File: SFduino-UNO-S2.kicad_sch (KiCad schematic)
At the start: 27 parts, among them J5 FPC 16p 0.5mm, SW1 SKHMQLE010, U1 SF32LB527UD6, U2 PY25Q128HA-WXH-IR, U8 CH334P, U9 CH343P, Y1 48M, Y2 12M

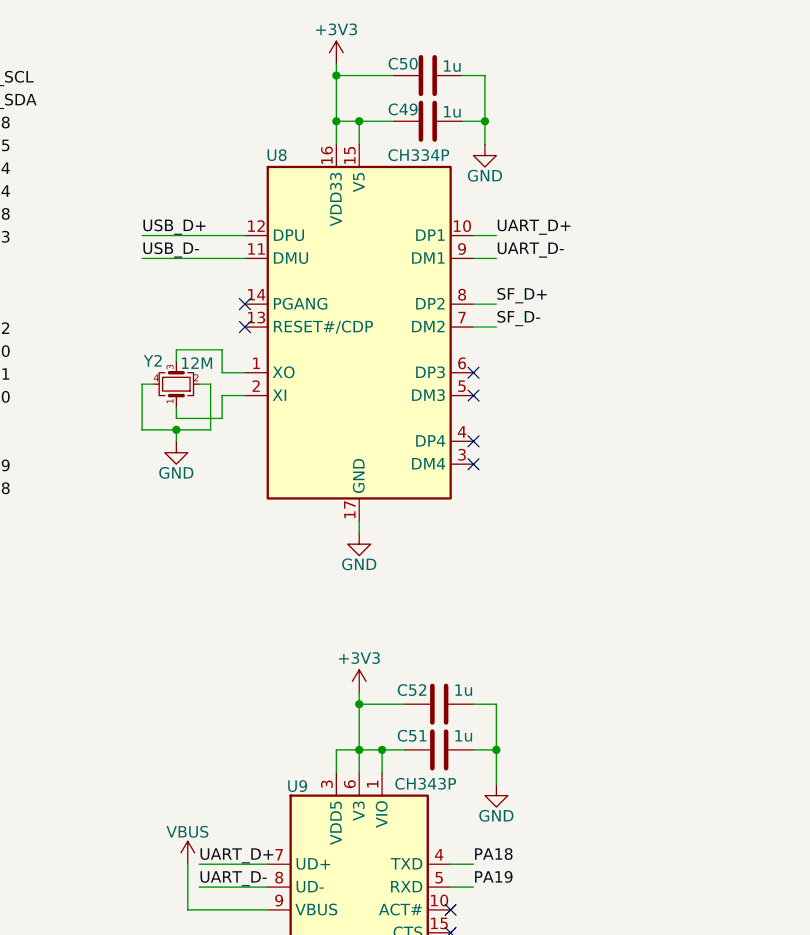
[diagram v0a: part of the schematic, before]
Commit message: fix: 修复电源架构
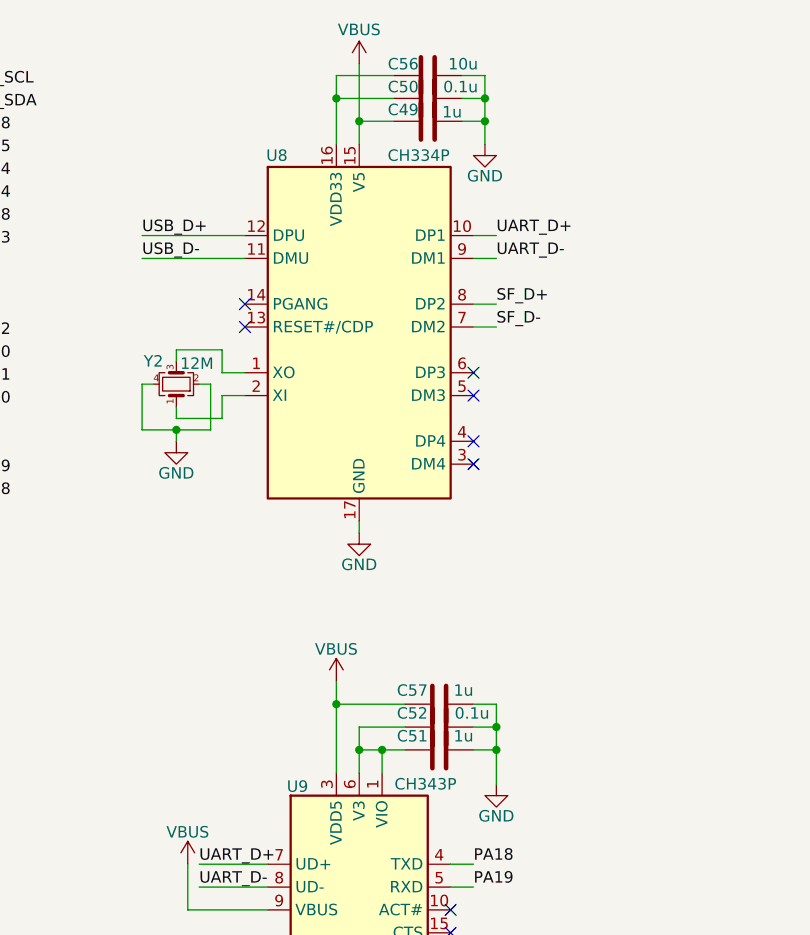
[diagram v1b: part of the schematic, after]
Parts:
- added C56: 10u, Capacitor_SMD:C_0402_1005Metric, symbol Device:C
- added C57: 1u, Capacitor_SMD:C_0402_1005Metric, symbol Device:C
- C50, C52: value 1u -> 0.1u
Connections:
- net GND: now also C56.2, C57.2
- net VBUS: now also C49.1, U8.15 (V5), U9.3 (VDD5), C57.1
- removed net +3V3: C49.1, C50.1, C51.1, C52.1, U8.15 (V5), U8.16 (VDD33), U9.1 (VIO), U9.3 (VDD5), U9.6 (V3)
- new net: C51.1, C52.1, U9.1 (VIO), U9.6 (V3)
- new net: C50.1, C56.1, U8.16 (VDD33)
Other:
- moved on the sheet: C50, C52
